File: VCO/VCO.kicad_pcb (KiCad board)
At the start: 2 copper layers, 162.2 x 104.5 mm, 151 parts, among them J101 Conn_02x05_Odd_Even, J201 AudioJack2_SwitchT, J202 AudioJack2_SwitchT, J203 AudioJack2_SwitchT, J204 AudioJack2_SwitchT, J301 AudioJack2_SwitchT, J401 AudioJack2_SwitchT, J402 AudioJack2_SwitchT, J501 AudioJack2_SwitchT, J502 AudioJack2_SwitchT, Q201 2N3906, Q202 2N3906, Q203 2N3904, Q204 2N3904, Q301 2N3904, Q302 2N3904, Q501 2N3904, Q502 2N3904, SW201 SW_SPDT, U101 TL072, U102 TL072, U103 TL072, U104 TL072, U105 TL072, U106 TL072, U107 TL072, U108 TL072, U109 TL072, U201 CA3080

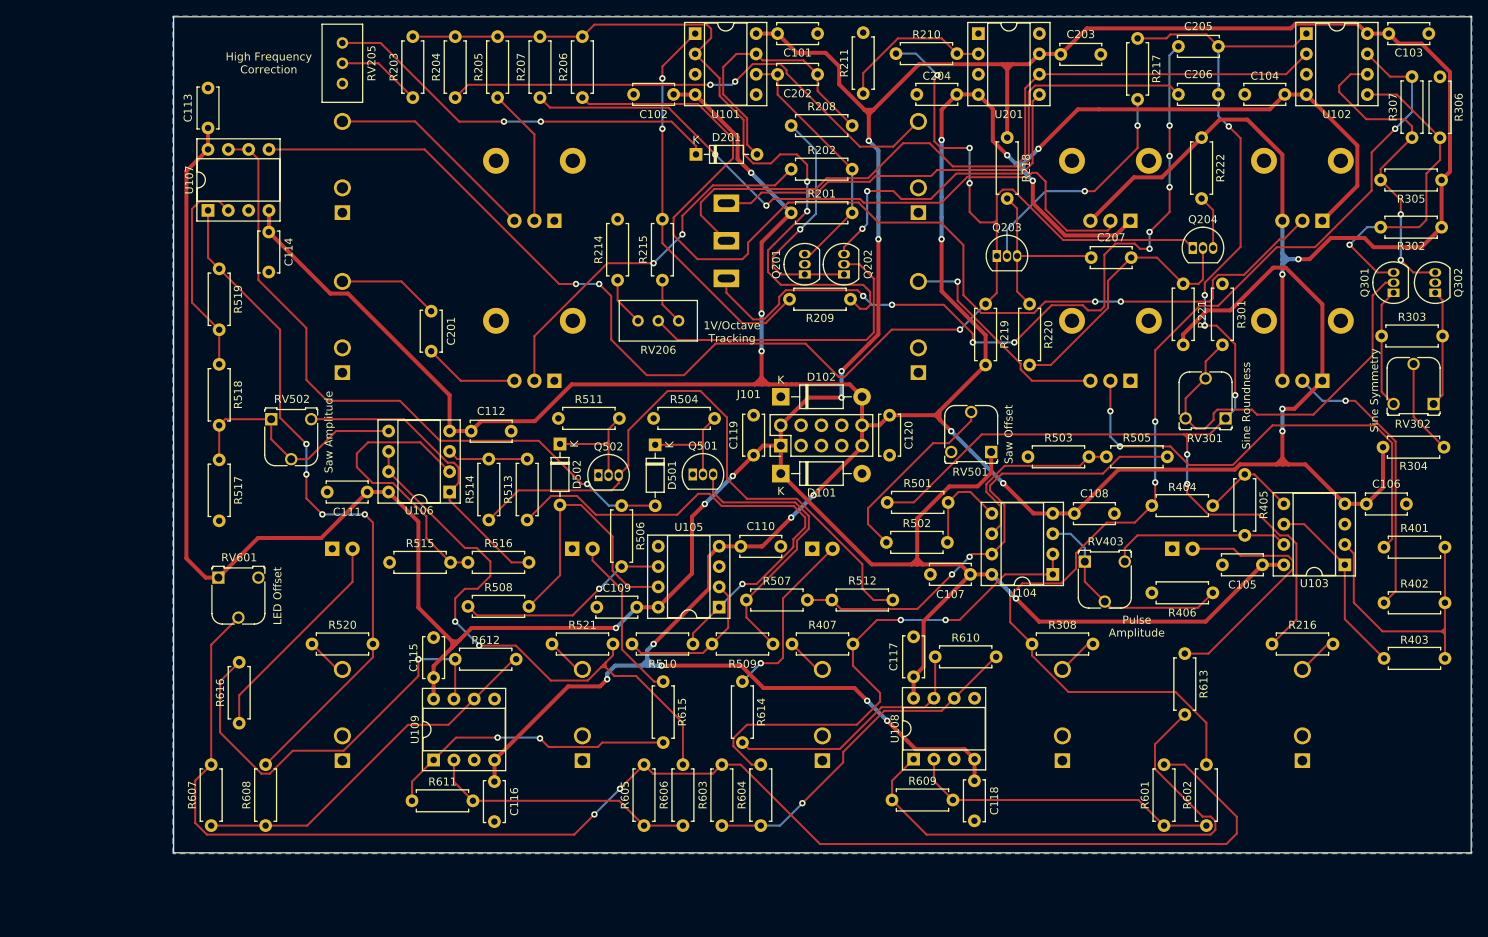
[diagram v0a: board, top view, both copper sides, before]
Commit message: Finish delay PCB
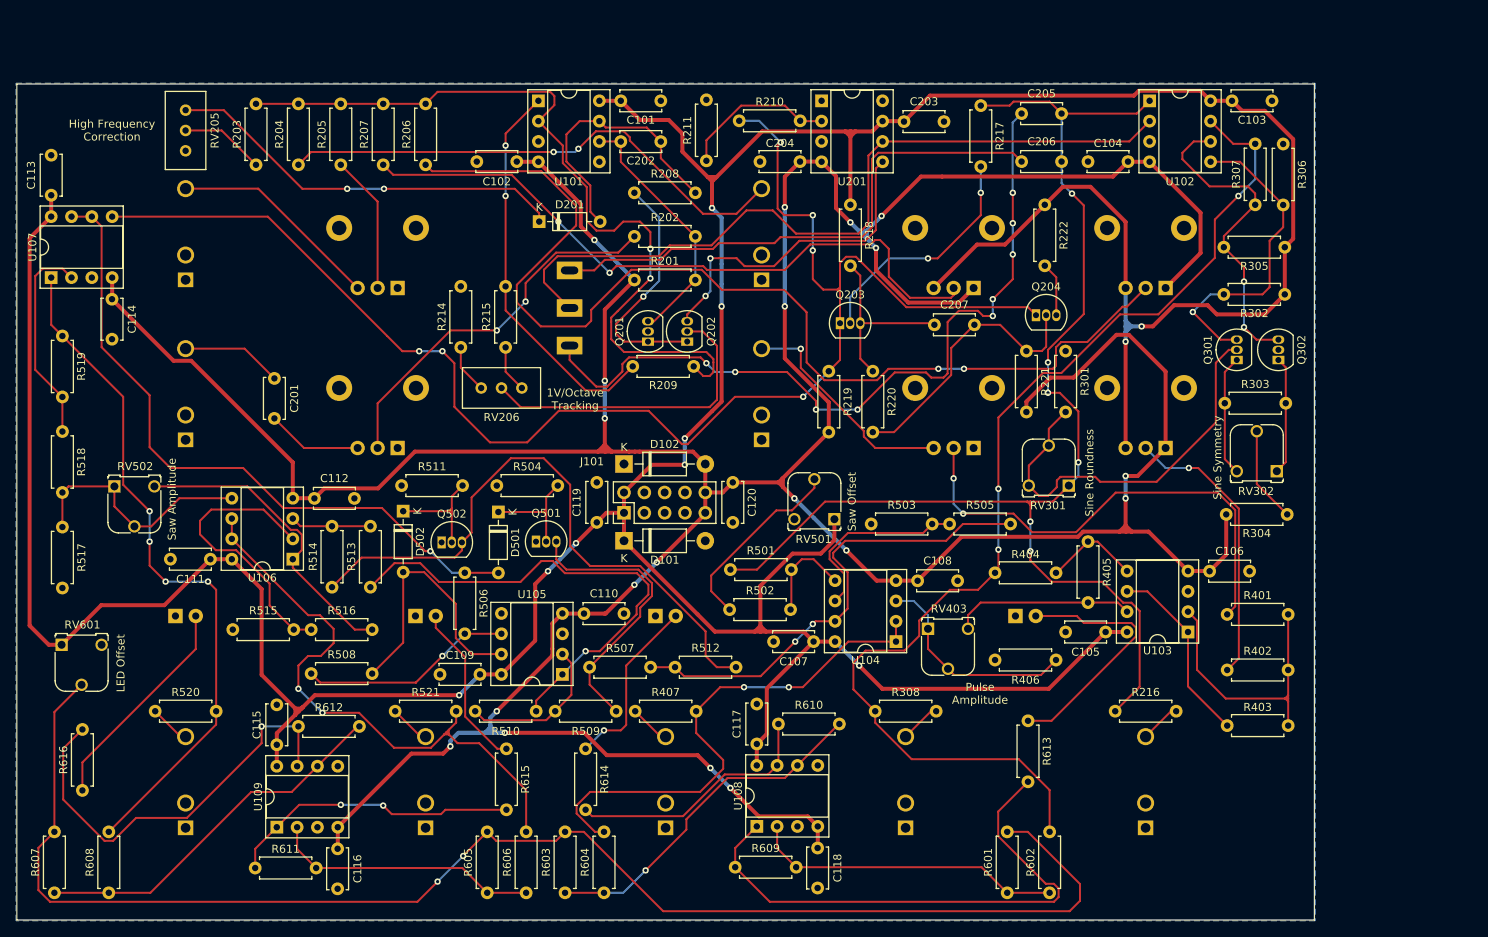
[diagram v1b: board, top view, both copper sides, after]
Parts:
- moved C207 21.3 mm to (179.7, 73.9)
- moved R221 21.3 mm to (191.2, 77.2)
- moved R403 21.3 mm to (223.9, 124.0)
- moved R501 21.3 mm to (154.2, 104.5)
- moved R509 21.3 mm to (139.9, 122.2)
- moved RV501 21.3 mm to (167.2, 98.2)
- moved R201 21.3 mm to (142.2, 68.3)
- moved R202 21.3 mm to (142.2, 62.9)
- moved R208 21.3 mm to (142.2, 57.4)
- moved R211 21.3 mm to (151.2, 53.4)
- moved R218 21.3 mm to (169.2, 58.9)
- moved U101 21.3 mm to (130.2, 45.9)
- moved Q302 21.3 mm to (222.7, 78.3)
- moved R610 21.3 mm to (160.2, 123.8)
- moved U105 21.3 mm to (133.2, 117.6)
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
